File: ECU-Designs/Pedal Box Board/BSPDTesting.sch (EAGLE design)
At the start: 16 parts, among them X1 MINIFIT_5566-2, X2 MINIFIT_5566-2

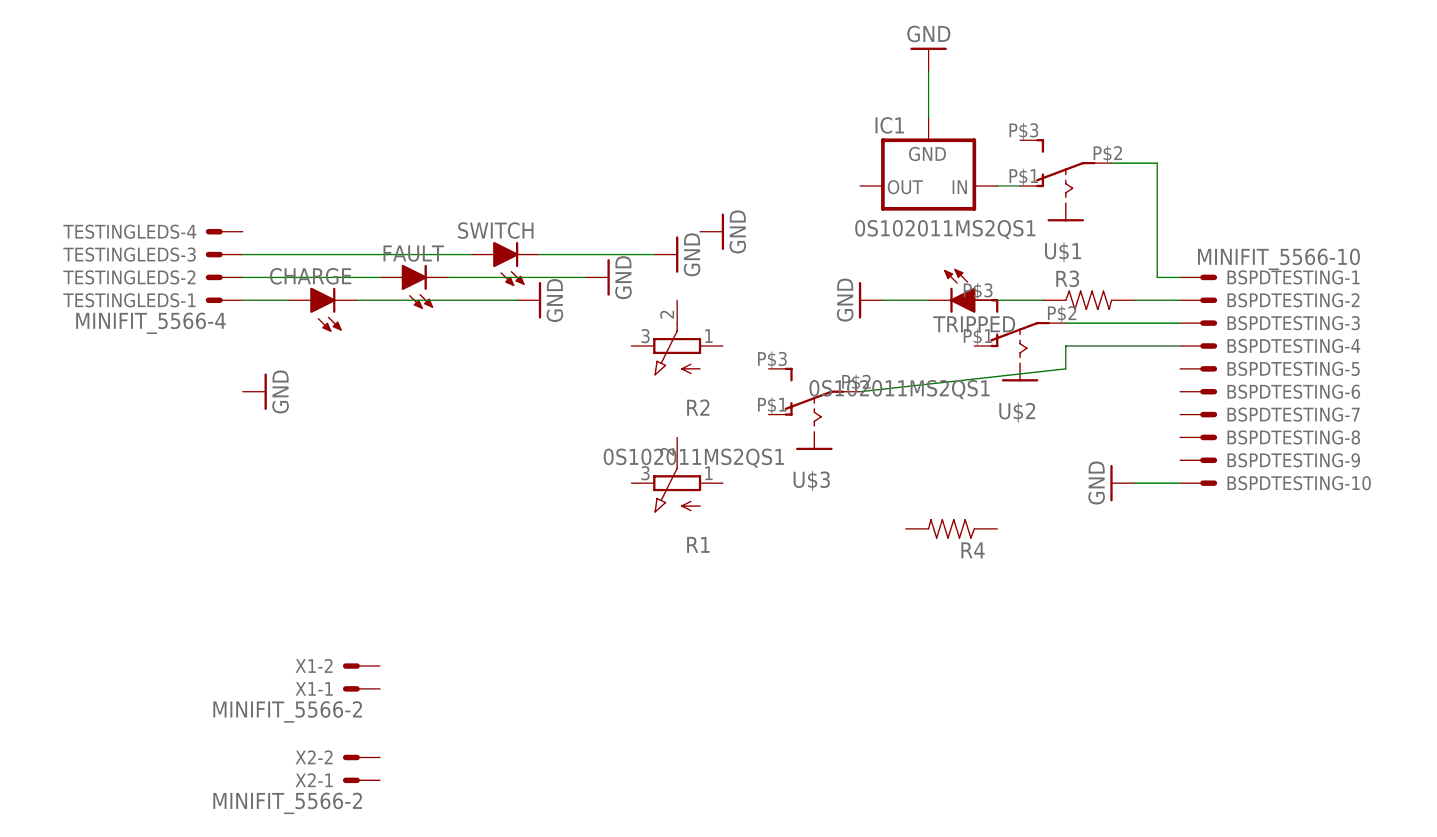
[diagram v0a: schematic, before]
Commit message: Cleaned up the schematic and made a board....are the LEDs fine?
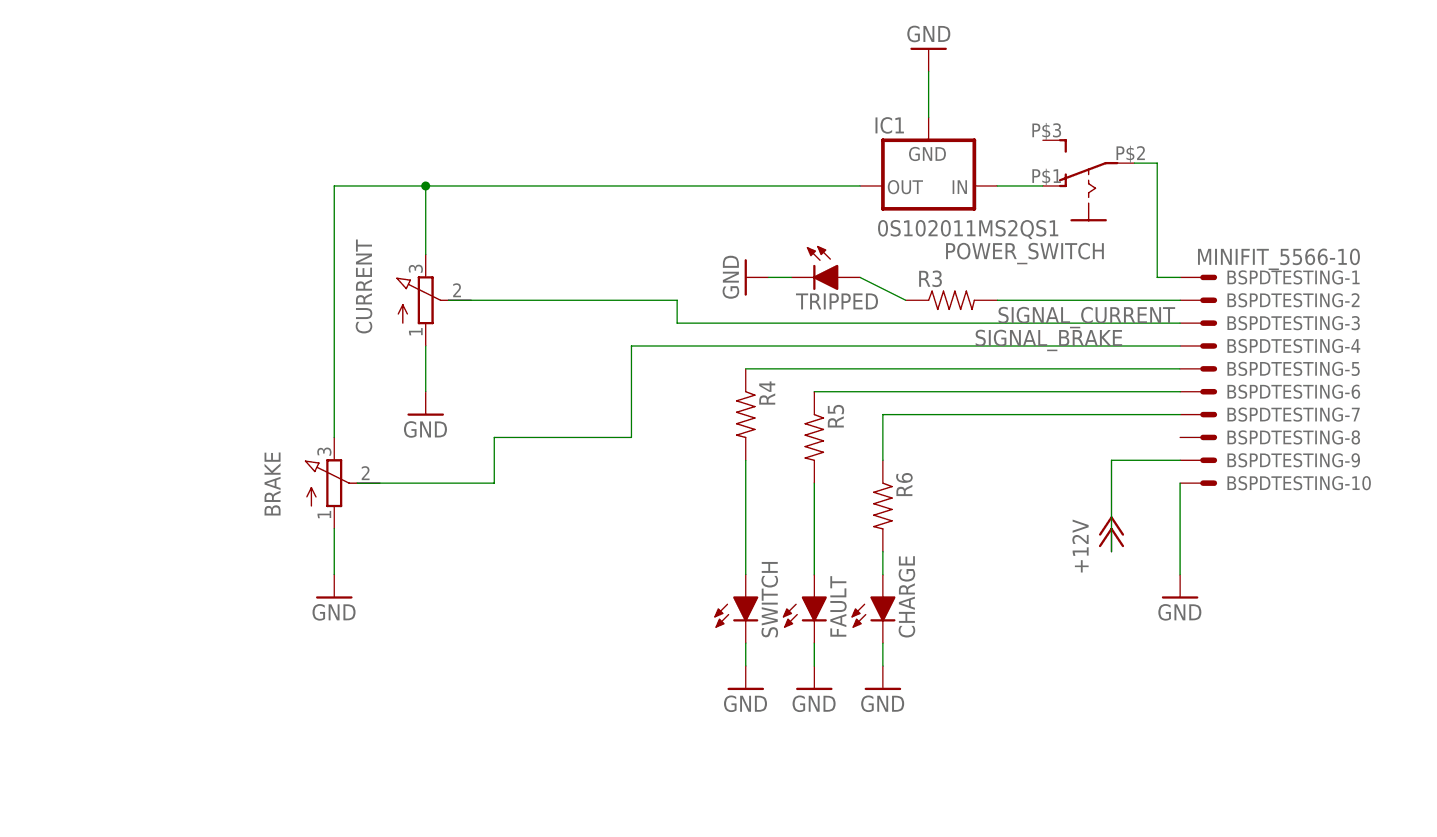
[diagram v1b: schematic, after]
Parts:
- removed R1, R2: (no value), HyTechDevices:3RP/1610N
- removed TESTINGLEDS: MINIFIT_5566-4, HyTechDevices:MINIFIT_5566-4
- removed U$1, U$2, U$3: 0S102011MS2QS1, HyTechDevices:0S102011MS2QS1
- removed X1, X2: MINIFIT_5566-2, HyTechDevices:MINIFIT_5566-2
- added BRAKE, CURRENT: (no value), HyTechDevices:3RP/1610N
- added POWER_SWITCH: 0S102011MS2QS1, HyTechDevices:0S102011MS2QS1
- added R5, R6: (no value), HyTechDevices:RESISTORAXIAL-0.3
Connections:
- removed net N$5: BSPDTESTING-3.S, U$2.P
- removed net N$6: BSPDTESTING-4.S, U$3.P
- new net +12V: BSPDTESTING-9.S
- new net N$12: R4.2, SWITCH.A
- new net N$13: CHARGE.A, R6.2
- new net N$14: BSPDTESTING-7.S, R6.1
- new net N$15: BRAKE.E, CURRENT.E, IC1.OUT
- new net SIGNAL_BRAKE: BSPDTESTING-4.S
- new net SIGNAL_CURRENT: BSPDTESTING-3.S
- net GND: now also BRAKE.A, CURRENT.A
- net N$1: now also POWER_SWITCH.P; no longer U$1.P
- net N$10: now also BSPDTESTING-6.S, R5.1; no longer SWITCH.A, TESTINGLEDS-3.S
- net N$4: now also POWER_SWITCH.O; no longer U$1.O
- net N$8: now also FAULT.A, R5.2; no longer CHARGE.A, TESTINGLEDS-1.S
- net N$9: now also BSPDTESTING-5.S, R4.1; no longer FAULT.A, TESTINGLEDS-2.S
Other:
- moved on the sheet: CHARGE, FAULT, R3, R4, SWITCH, TRIPPED
